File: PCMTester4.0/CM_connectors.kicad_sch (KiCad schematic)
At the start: 28 parts, among them J2 FX11A-80P8, J3 FX11A-80P8

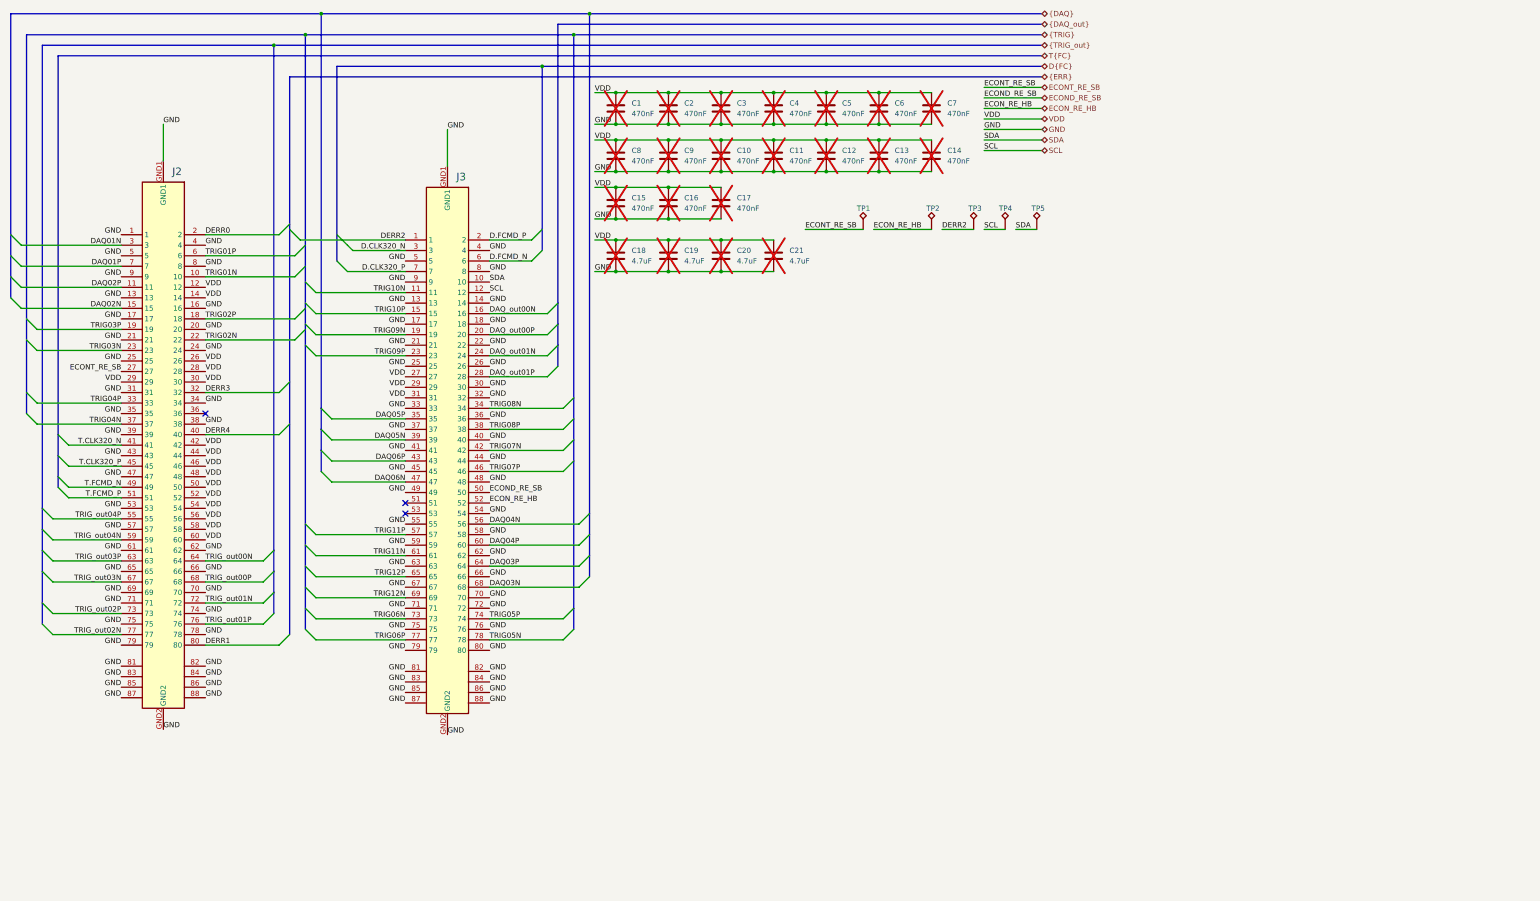
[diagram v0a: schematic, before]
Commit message: FINAL VERSION
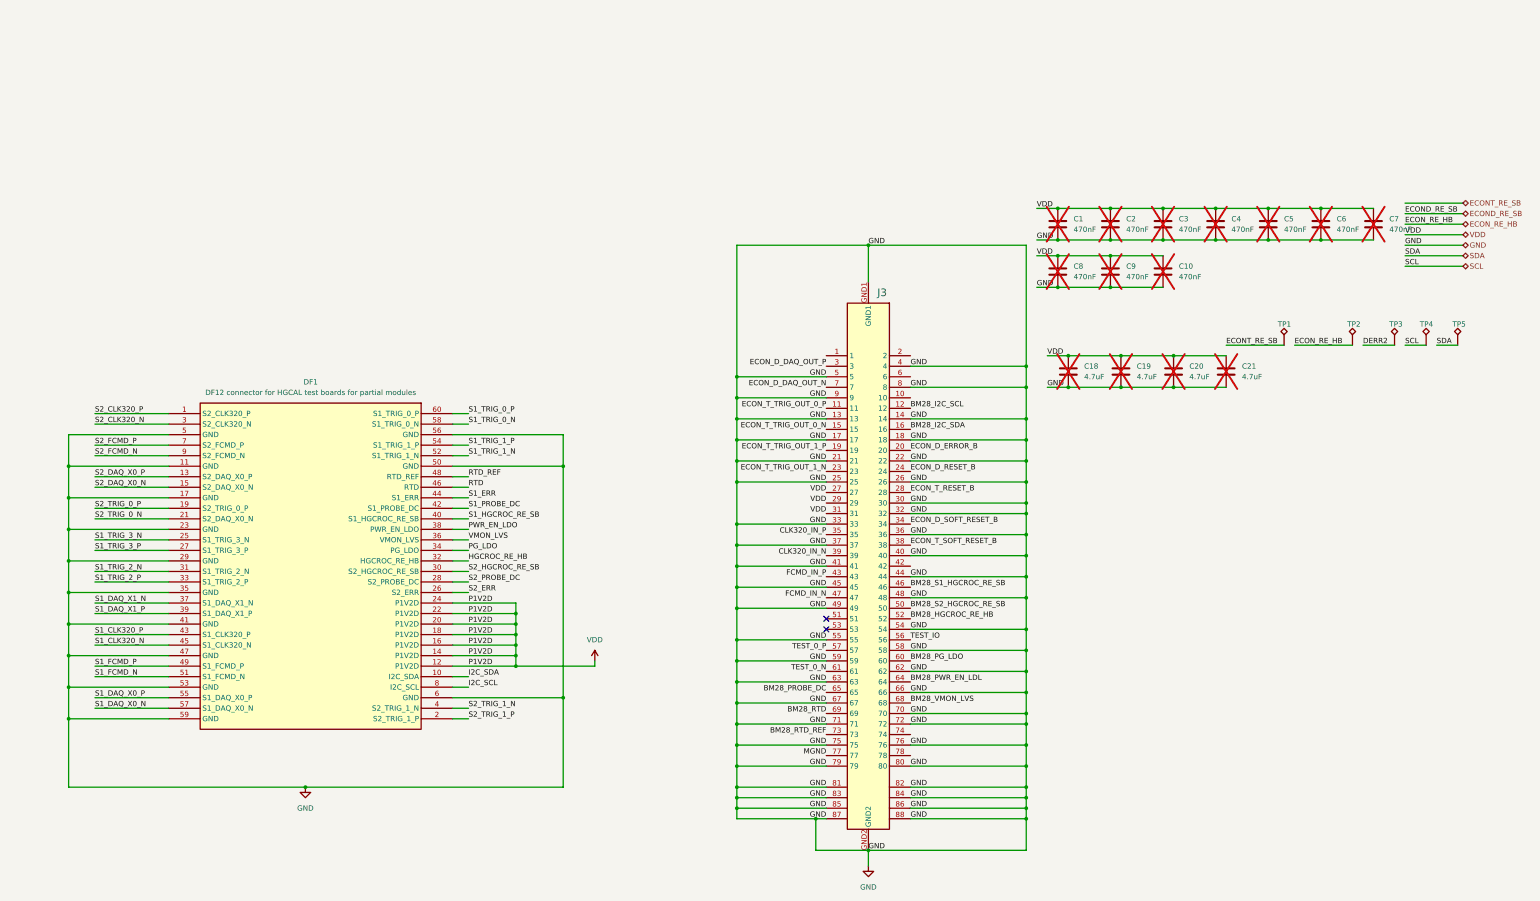
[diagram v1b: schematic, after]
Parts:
- removed C11, C12, C13, C14, C15, C16, C17: 470nF, Capacitor_SMD:C_0402_1005Metric, symbol Device:C
- removed J2: FX11A-80P8, Library:HIROSE_FX11A-80P-8-SV, symbol ECON:FX11A-80P8
- added DF1: DF12 connector for HGCAL test boards for partial 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, PCMFootprints:HRS_DF12NB-60DS-0.5V_51_, symbol DF12_symbol.schlib:root_0_DF12NB-60DS-0.5V_pCM_test.SCHLIB
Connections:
- net DERR2: no longer J3.1
- net ECOND_RE_SB: no longer J3.50
- net ECON_RE_HB: no longer J3.52
- net GND: now also DF1.11 (GND), DF1.17 (GND), DF1.23 (GND), DF1.29 (GND), DF1.35 (GND), DF1.41 (GND), DF1.47 (GND), DF1.5 (GND), DF1.50 (GND), DF1.53 (GND), DF1.56 (GND), DF1.59 (GND), DF1.6 (GND)
- net SCL: no longer J3.12
- net SDA: no longer J3.10
- net VDD: now also DF1.12 (P1V2D), DF1.14 (P1V2D), DF1.16 (P1V2D), DF1.18 (P1V2D), DF1.20 (P1V2D), DF1.22 (P1V2D), DF1.24 (P1V2D)
- net D.CLK320_N renamed ECON_D_DAQ_OUT_P
- net D.CLK320_P renamed ECON_D_DAQ_OUT_N
- net D.FCMD_N: no longer names the net of J3.6
- net D.FCMD_P: no longer names the net of J3.2
- net DAQ03N renamed BM28_VMON_LVS
- net DAQ03P renamed BM28_PWR_EN_LDL
- net DAQ04N renamed TEST_IO
- net DAQ04P renamed BM28_PG_LDO
- net DAQ05N renamed CLK320_IN_N
- net DAQ05P renamed CLK320_IN_P
- net DAQ06N renamed FCMD_IN_N
- net DAQ06P renamed FCMD_IN_P
- net DAQ_out00N renamed BM28_I2C_SDA
- net DAQ_out00P renamed ECON_D_ERROR_B
- net DAQ_out01N renamed ECON_D_RESET_B
- net DAQ_out01P renamed ECON_T_RESET_B
- net TRIG05N: no longer names the net of J3.78
- net TRIG05P: no longer names the net of J3.74
- net TRIG06N renamed BM28_RTD_REF
- net TRIG06P renamed MGND
- net TRIG07N: no longer names the net of J3.42
- net TRIG07P renamed BM28_S1_HGCROC_RE_SB
- net TRIG08N renamed ECON_D_SOFT_RESET_B
- net TRIG08P renamed ECON_T_SOFT_RESET_B
- net TRIG09N renamed ECON_T_TRIG_OUT_1_P
- net TRIG09P renamed ECON_T_TRIG_OUT_1_N
- net TRIG10N renamed ECON_T_TRIG_OUT_0_P
- net TRIG10P renamed ECON_T_TRIG_OUT_0_N
- net TRIG11N renamed TEST_0_N
- net TRIG11P renamed TEST_0_P
- net TRIG12N renamed BM28_RTD
- net TRIG12P renamed BM28_PROBE_DC
- new net BM28_HGCROC_RE_HB: J3.52
- new net BM28_I2C_SCL: J3.12
- new net BM28_S2_HGCROC_RE_SB: J3.50
- new net HGCROC_RE_HB: DF1.32 (HGCROC_RE_HB)
- new net I2C_SCL: DF1.8 (I2C_SCL)
- new net I2C_SDA: DF1.10 (I2C_SDA)
- new net PG_LDO: DF1.34 (PG_LDO)
- new net PWR_EN_LDO: DF1.38 (PWR_EN_LDO)
- new net RTD: DF1.46 (RTD)
- new net RTD_REF: DF1.48 (RTD_REF)
- new net S1_CLK320_N: DF1.45 (S1_CLK320_N)
- new net S1_CLK320_P: DF1.43 (S1_CLK320_P)
- new net S1_DAQ_X0_N: DF1.57 (S1_DAQ_X0_N)
- new net S1_DAQ_X0_P: DF1.55 (S1_DAQ_X0_P)
- new net S1_DAQ_X1_N: DF1.37 (S1_DAQ_X1_N)
- new net S1_DAQ_X1_P: DF1.39 (S1_DAQ_X1_P)
- new net S1_ERR: DF1.44 (S1_ERR)
- new net S1_FCMD_N: DF1.51 (S1_FCMD_N)
- new net S1_FCMD_P: DF1.49 (S1_FCMD_P)
- new net S1_HGCROC_RE_SB: DF1.40 (S1_HGCROC_RE_SB)
- new net S1_PROBE_DC: DF1.42 (S1_PROBE_DC)
- new net S1_TRIG_0_N: DF1.58 (S1_TRIG_0_N)
- new net S1_TRIG_0_P: DF1.60 (S1_TRIG_0_P)
- new net S1_TRIG_1_N: DF1.52 (S1_TRIG_1_N)
- new net S1_TRIG_1_P: DF1.54 (S1_TRIG_1_P)
- new net S1_TRIG_2_N: DF1.31 (S1_TRIG_2_N)
- new net S1_TRIG_2_P: DF1.33 (S1_TRIG_2_P)
- new net S1_TRIG_3_N: DF1.25 (S1_TRIG_3_N)
- new net S1_TRIG_3_P: DF1.27 (S1_TRIG_3_P)
- new net S2_CLK320_N: DF1.3 (S2_CLK320_N)
- new net S2_CLK320_P: DF1.1 (S2_CLK320_P)
- new net S2_DAQ_X0_N: DF1.15 (S2_DAQ_X0_N)
- new net S2_DAQ_X0_P: DF1.13 (S2_DAQ_X0_P)
- new net S2_ERR: DF1.26 (S2_ERR)
- new net S2_FCMD_N: DF1.9 (S2_FCMD_N)
- new net S2_FCMD_P: DF1.7 (S2_FCMD_P)
- new net S2_HGCROC_RE_SB: DF1.30 (S2_HGCROC_RE_SB)
- new net S2_PROBE_DC: DF1.28 (S2_PROBE_DC)
- new net S2_TRIG_0_N: DF1.21 (S2_DAQ_X0_N)
- new net S2_TRIG_0_P: DF1.19 (S2_TRIG_0_P)
- new net S2_TRIG_1_N: DF1.4 (S2_TRIG_1_N)
- new net S2_TRIG_1_P: DF1.2 (S2_TRIG_1_P)
- new net VMON_LVS: DF1.36 (VMON_LVS)
- no-connect marks 3 -> 2
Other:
- moved on the sheet: C1, C10, C18, C19, C2, C20, C21, C3, C4, C5, C6, C7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

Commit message: ts buss
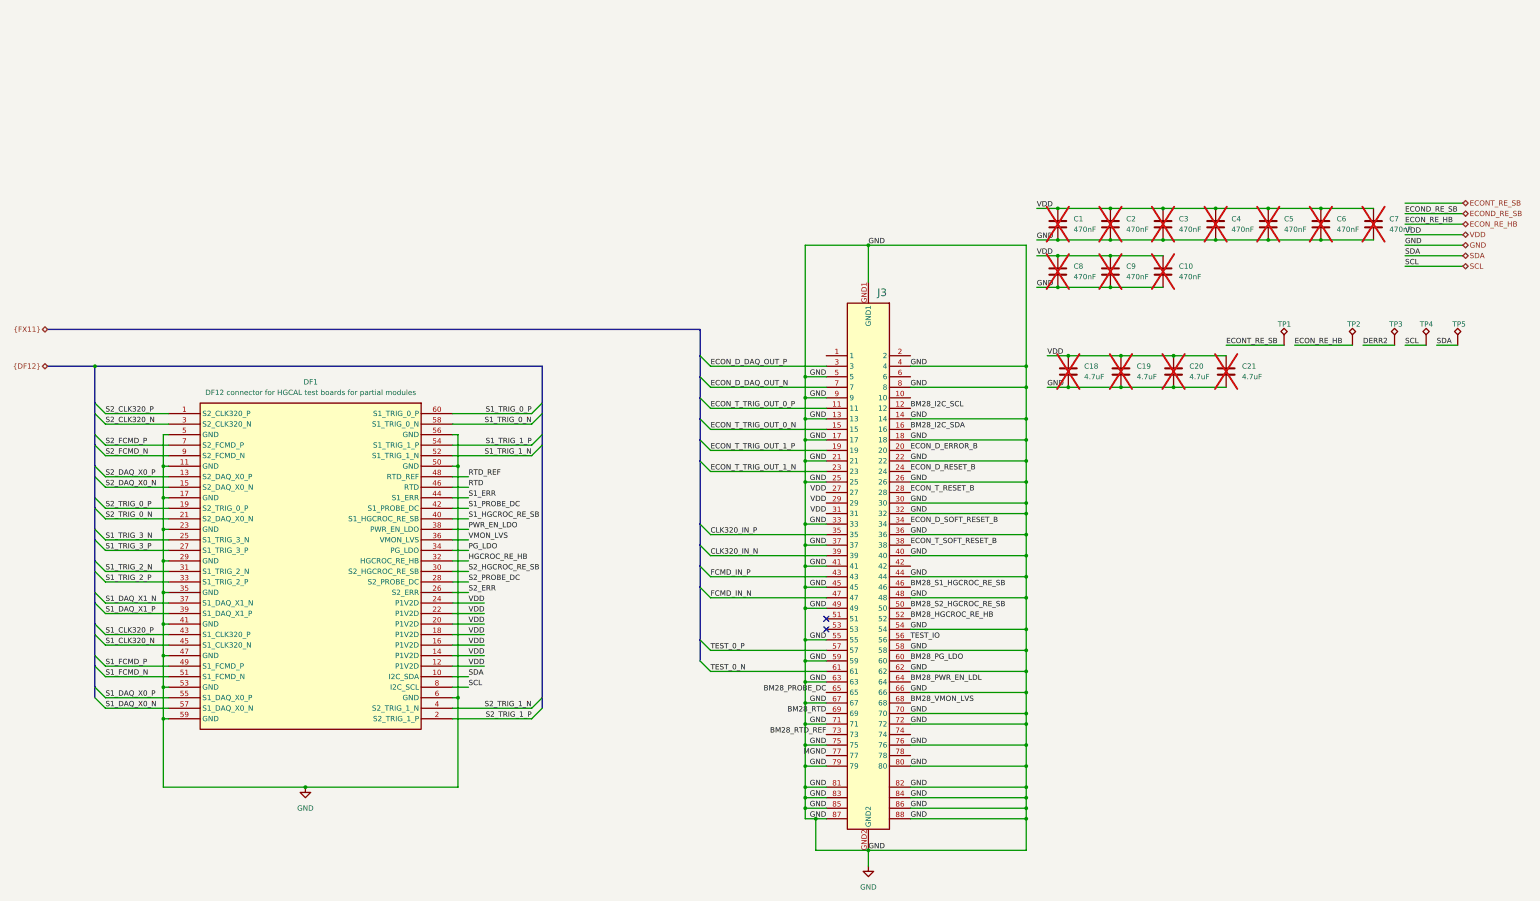
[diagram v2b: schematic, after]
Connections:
- net I2C_SCL is gone; now on net SCL: DF1.8 (I2C_SCL)
- net I2C_SDA is gone; now on net SDA: DF1.10 (I2C_SDA)
